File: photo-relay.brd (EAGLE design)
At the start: 40 x 45 mm, 11 parts, among them IC1 LM393N, K1 351, Q1 2N3565, X1 MKDSN1,5/3-5,08, X2 MKDSN1,5/2-5,08

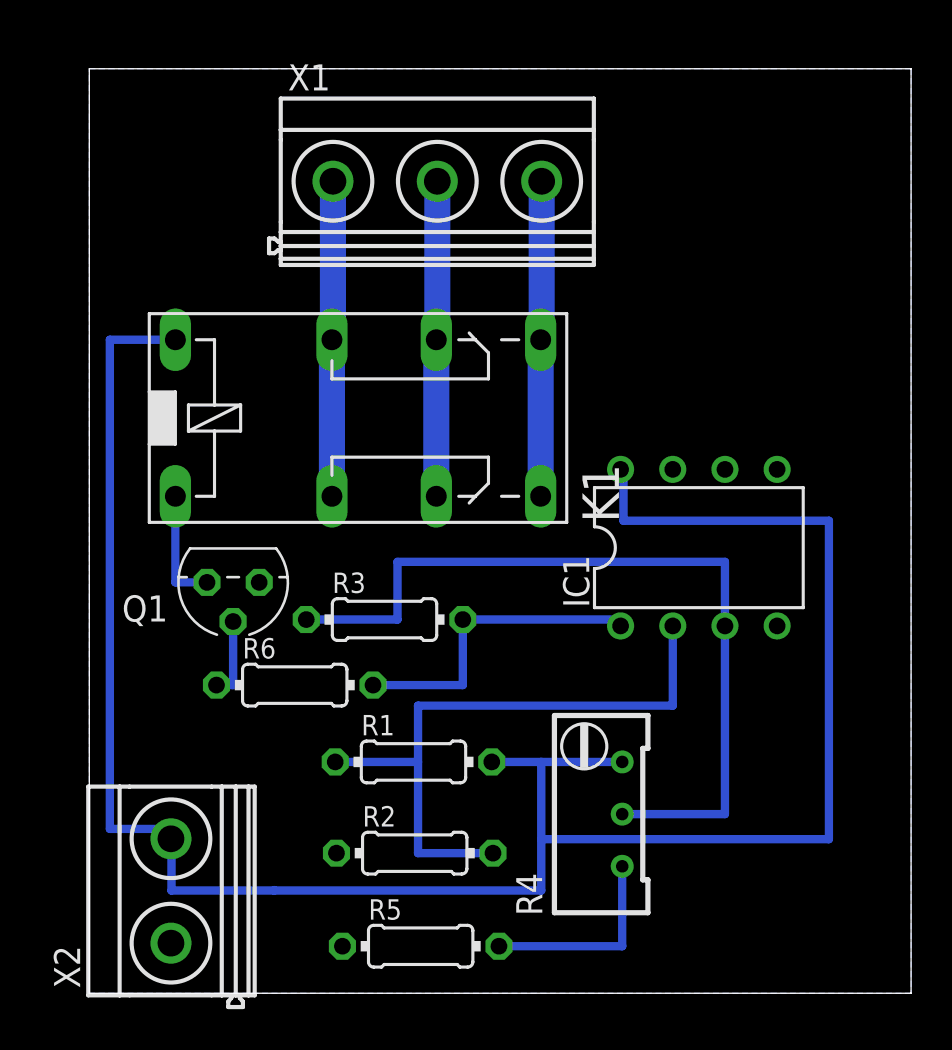
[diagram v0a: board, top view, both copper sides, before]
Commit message: minor changes
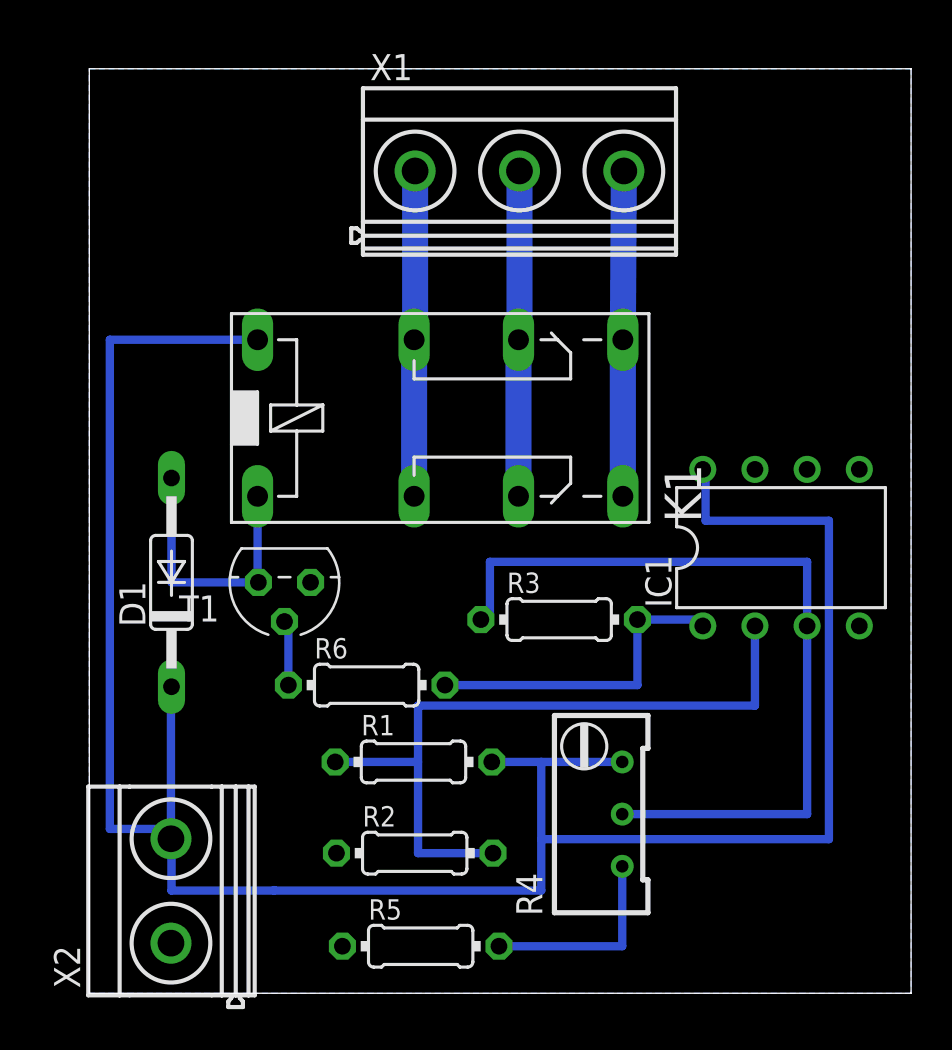
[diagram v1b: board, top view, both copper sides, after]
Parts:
- removed Q1: 2N3565, transistor-npn:TO92
- added D1: 1N4148DO35-10, diode:DO35-10
- added T1: 2N3904, transistor:TO92
- R6: value 1K -> 10K
- moved R3 8.50 mm to (22.9, 18.2)
- moved X1 4.03 mm to (23.5, 40.0)
- moved IC1 4.00 mm to (33.7, 21.7)
- moved K1 4.00 mm to (12.0, 28.0)
- moved R6 3.50 mm to (13.5, 15.0)
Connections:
- net GND: now also T1.3; no longer Q1.3
- net N$5: now also T1.2; no longer Q1.2
- net N$7: now also D1.A, T1.1; no longer Q1.1
- net V+: now also D1.C
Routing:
- net N$7: track 5.73 -> 13.5 mm
- net V+: track 105.8 -> 113.2 mm
- net N$4: track 31.1 -> 35.1 mm
- net N$1: track 15.6 -> 16.1 mm
- net N$8: track 15.4 -> 15.9 mm
- net N$2: track 40.5 -> 40.0 mm
- net N$10: track 15.4 -> 15.9 mm
